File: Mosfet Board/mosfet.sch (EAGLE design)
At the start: 8 parts

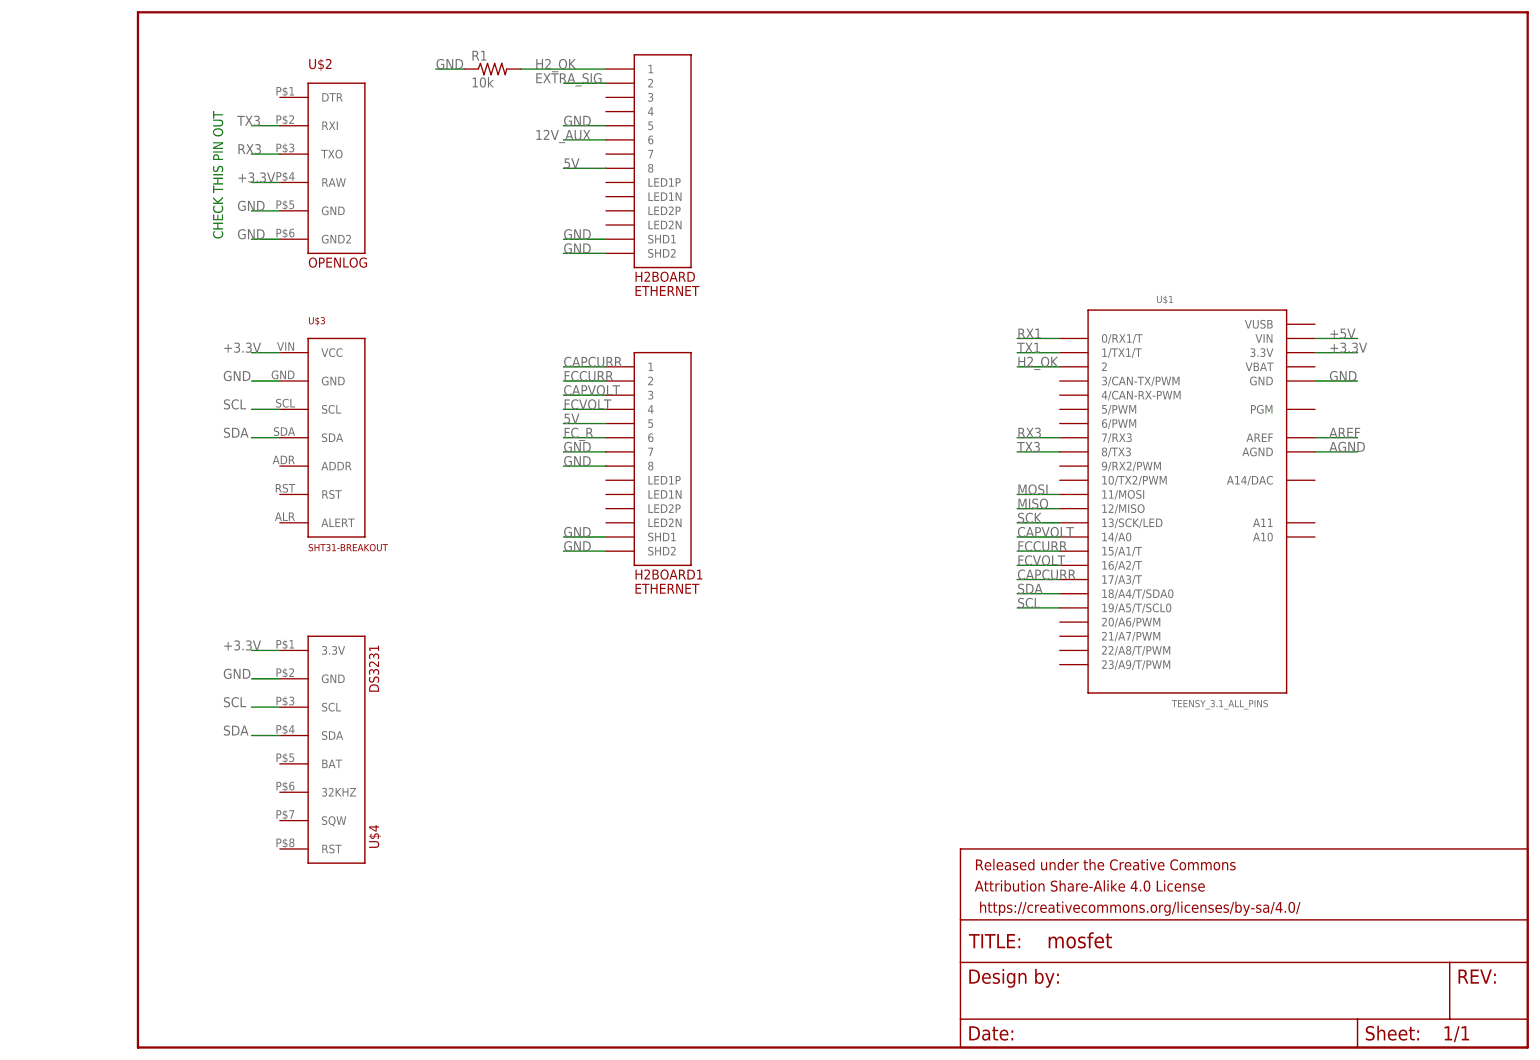
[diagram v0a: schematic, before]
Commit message: update
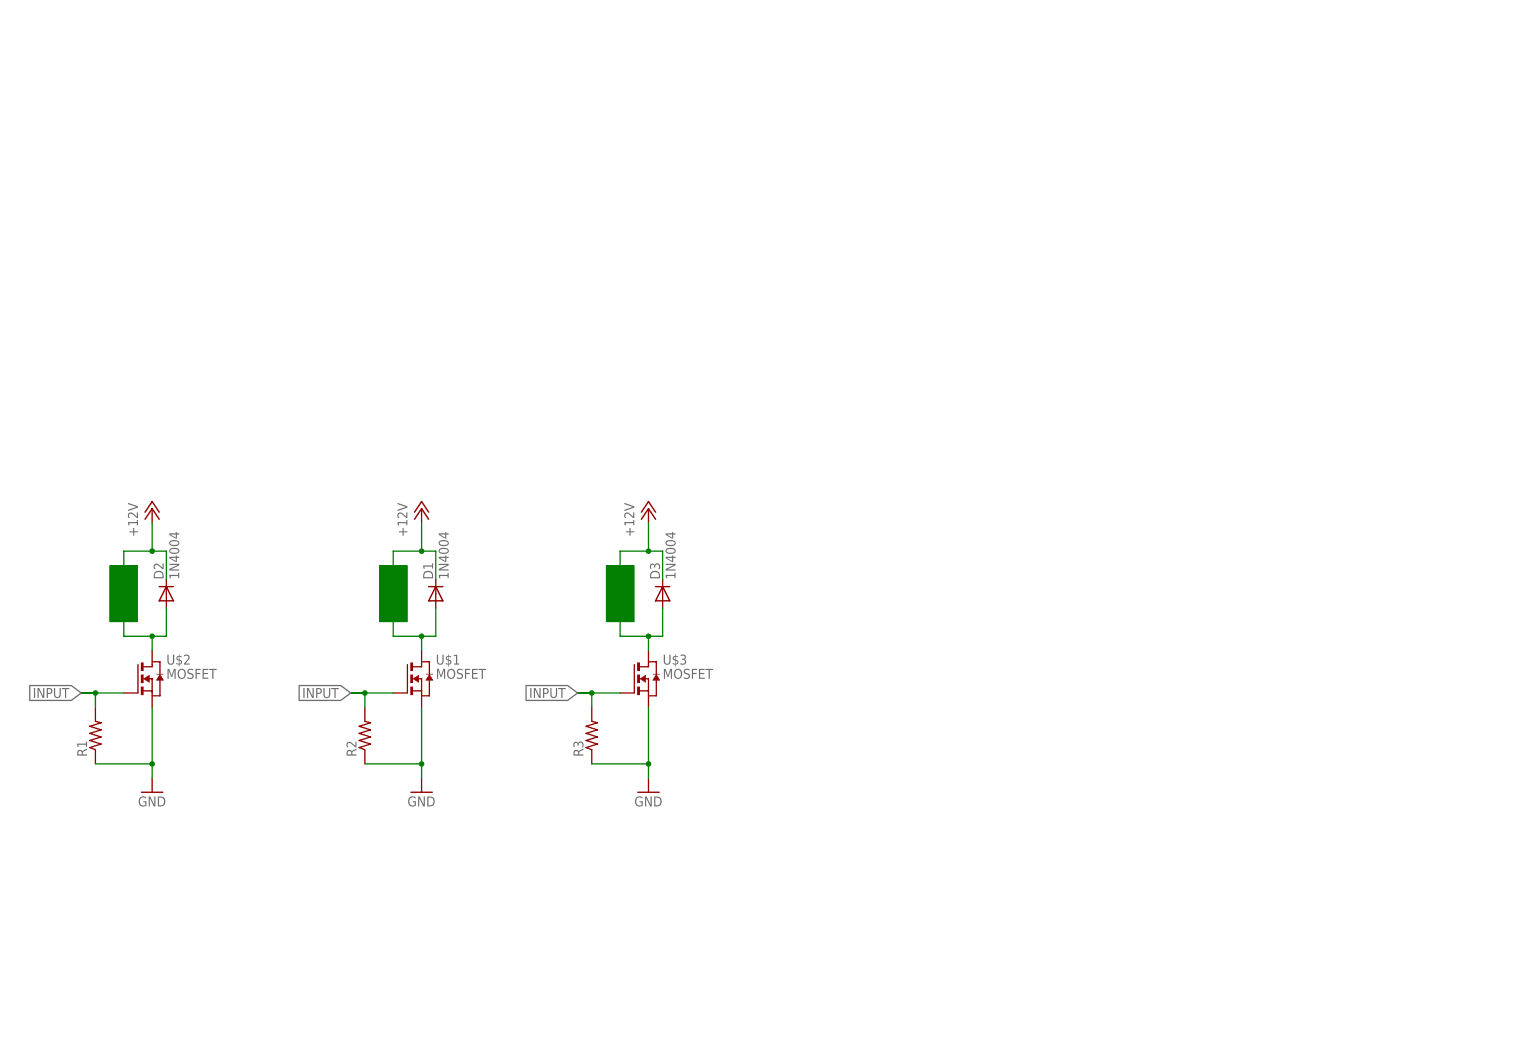
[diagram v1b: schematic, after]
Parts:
- removed FRAME1: FRAME-LETTERNO_PACKAGE, SparkFun-Aesthetics:FRAME-LETTERNO_PACKAGE
- removed H2BOARD, H2BOARD1: ETHERNET, ETHERNET:ETHERNET
- removed U$4: DS3231, DS3231:DS3231
- added D1, D2, D3: 1N4004, diode:1N4004
- added R2, R3: (no value), resistor:R-US_R0603
- R1: value 10k -> (none); device adafruit:R-US_R0603 -> resistor:R-US_R0603
- U$1: value TEENSY_3.1_ALL_PINS -> MOSFET; device Teensy_3_and_LC_Series_Boards_v1.1:TEENSY_3.1_ALL_PINS -> MOSFET:MOSFET
- U$2: value OPENLOG -> MOSFET; device openlog:OPENLOG -> MOSFET:MOSFET
- U$3: value SHT31-BREAKOUT -> MOSFET; device SHT31Breakout:SHT31-BREAKOUT -> MOSFET:MOSFET
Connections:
- removed net +3.3V: U$1.3.3V, U$2.RAW, U$3.VCC, U$4.3.3V
- removed net +5V: U$1.VIN
- removed net 12V_AUX: H2BOARD.6
- removed net 5V: H2BOARD.8, H2BOARD1.5
- removed net AGND: U$1.AGND
- removed net AREF: U$1.AREF
- removed net CAPCURR: H2BOARD1.1, U$1.17/A3/T
- removed net CAPVOLT: H2BOARD1.3, U$1.14/A0
- removed net EXTRA_SIG: H2BOARD.2
- removed net FCCURR: H2BOARD1.2, U$1.15/A1/T
- removed net FCVOLT: H2BOARD1.4, U$1.16/A2/T
- removed net FC_R: H2BOARD1.6
- removed net H2_OK: H2BOARD.1, R1.2, U$1.2
- removed net MISO: U$1.12/MISO
- removed net MOSI: U$1.11/MOSI
- removed net RX1: U$1.0/RX1/T
- removed net RX3: U$1.7/RX3, U$2.TXO
- removed net SCK: U$1.13/SCK/LED
- removed net SCL: U$1.19/A5/T/SCL0, U$3.SCL, U$4.SCL
- removed net SDA: U$1.18/A4/T/SDA0, U$3.SDA, U$4.SDA
- removed net TX1: U$1.1/TX1/T
- removed net TX3: U$1.8/TX3, U$2.RXI
- new net +12V: D1.C, D2.C, D3.C
- new net N$1: R2.2, U$1.G
- new net N$2: D1.A, U$1.D
- new net N$3: D2.A, U$2.D
- new net N$4: R1.2, U$2.G
- new net N$5: D3.A, U$3.D
- new net N$6: R3.2, U$3.G
- net GND: now also R2.1, R3.1, U$1.S, U$2.S, U$3.S; no longer H2BOARD.5, H2BOARD.SHD1, H2BOARD.SHD2, H2BOARD1.7, H2BOARD1.8, H2BOARD1.SHD1, H2BOARD1.SHD2, U$1.GND, U$2.GND, U$2.GND2, U$3.GND, U$4.GND
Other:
- note removed: "CHECK THIS PIN OUT"
- moved on the sheet: R1
